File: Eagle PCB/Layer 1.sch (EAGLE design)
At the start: 231 parts, among them M1C1 33nF, M1C2 680uF, M1C3 1.0uF, M1D1 RED, M1D2 BLUE, M1J1 XT30PB-F, M1Q1 AOD482, M1R1 1k, M1R10 1k, M1R11 10k, M1R12 4.7k, M1R2 1k, M1R3 3.3k, M1R4 3.3k, M1R5 1k, M1R6 1k, M1R7 1k, M1R8 10k, M1R9 10k, M2C1 33nF, M2C2 680uF, M2C3 1.0uF, M2D1 RED, M2D2 BLUE, M2J1 XT30PB-F, M2Q1 AOD482, M2R1 1k, M2R10 1k, M2R11 10k, M2R12 4.7k, M2R2 1k, M2R3 3.3k, M2R4 3.3k, M2R5 1k, M2R6 1k, M2R7 1k, M2R8 10k, M2R9 10k, M3C1 33nF, M3C2 680uF, M3C3 1.0uF, M3D1 RED, M3D2 BLUE, M3J1 XT30PB-F, M3Q1 AOD482, M3R1 1k, M3R10 1k, M3R11 10k, M3R12 4.7k, M3R2 1k, M3R3 3.3k, M3R4 3.3k, M3R5 1k, M3R6 1k, M3R7 1k, M3R8 10k, M3R9 10k, M4C1 33nF, M4C2 680uF, M4C3 1.0uF, M4D1 RED, M4D2 BLUE, M4J1 XT30PB-F, M4Q1 AOD482, M4R1 1k, M4R10 1k, M4R11 10k, M4R12 4.7k, M4R2 1k, M4R3 3.3k, M4R4 3.3k, M4R5 1k, M4R6 1k, M4R7 1k, M4R8 10k, M4R9 10k, Q1 LIGHT_SENSORALS, Q10 LIGHT_SENSORALS, Q11 LIGHT_SENSORALS, Q12 LIGHT_SENSORALS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

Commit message: FUCK YOU
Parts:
- added 1C10: 22uF, JH:CAPACITOR1210
- added 1C6: 4.7uF, JH:CAPACITOR0603
- added 1C7: 220uF, SparkFun-Capacitors:100UF-POLAR-EIA7343-10V-10%(TANT)
- added 1C8: 10nF, JH:CAPACITOR0603
- added 1C9: 0.1uF, JH:CAPACITOR0603
- added 1D2: SS54, JH:DIODE-SCHOTTKY
- added 1L2: 10uH, JH:INDUCTORSWPA8040
- added 1R3: 10k, JH:RESISTOR0603
- added 1R4: 3.24k, JH:RESISTOR0603
- added BATT: XT30PB-F, JH:XT30PB-F
- added U2: (no value), JH:TPS54X0
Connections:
- new net 5V: 1C7.+, 1C9.1, 1L2.2, 1R3.2
- new net N$3: 1C8.2, 1D2.C, 1L2.1, U2.PH
- new net N$5: 1R3.1, 1R4.2, U2.VSNS
- new net N$6: 1C8.1, U2.BOOT
- net GND: now also 1C10.2, 1C6.2, 1C7.-, 1C9.2, 1D2.A, 1R4.1, BATT.P$V-, U2.GND
- net V_BATT: now also 1C10.1, 1C6.1, BATT.P$V+, U2.VIN
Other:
- note added: "5V BUCK"

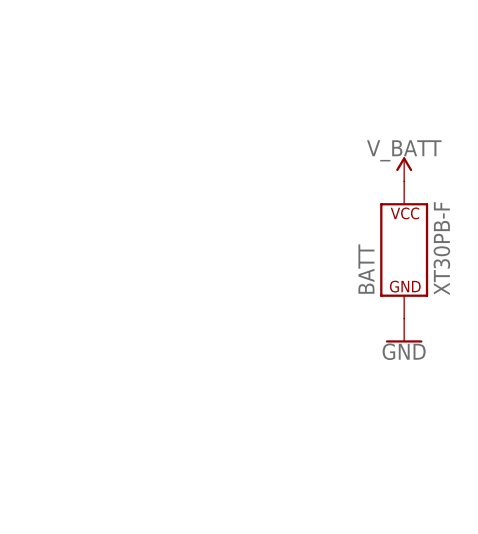
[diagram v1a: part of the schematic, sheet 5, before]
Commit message: Hello
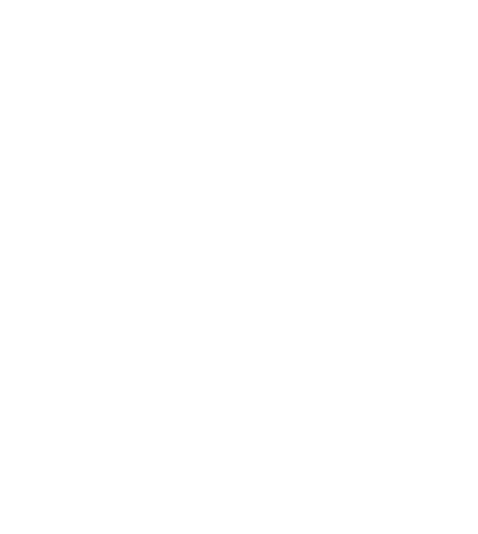
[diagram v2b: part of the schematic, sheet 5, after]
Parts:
- removed BATT: XT30PB-F, JH:XT30PB-F
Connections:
- net GND: no longer BATT.P$V-
- net V_BATT: no longer BATT.P$V+
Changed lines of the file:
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@@
 <part name="V_BATT_M4B" library="JH" library_urn="urn:adsk.eagle:library:6027132" deviceset="18AWG" device="" package3d_urn="urn:adsk.eagle:package:16754415/1"/>
 <part name="FRAME2" library="SparkFun-Aesthetics" deviceset="FRAME-A4L" device=""/>
-<part name="SUPPLY3" library="SparkFun-PowerSymbols" deviceset="V_BATT" device=""/>
-<part name="GND16" library="SparkFun-PowerSymbols" deviceset="GND" device=""/>
 <part name="SUPPLY22" library="SparkFun-PowerSymbols" deviceset="V_BATT" device=""/>
 <part name="1C6" library="JH" library_urn="urn:adsk.eagle:library:6027132" deviceset="CAPACITOR" device="0603" package3d_urn="urn:adsk.eagle:package:15441226/3" value="4.7uF"/>
@@
 <part name="1C9" library="JH" library_urn="urn:adsk.eagle:library:6027132" deviceset="CAPACITOR" device="0603" package3d_urn="urn:adsk.eagle:package:15441226/3" value="0.1uF"/>
 <part name="SUPPLY28" library="SparkFun-PowerSymbols" deviceset="5V" device=""/>
-<part name="BATT" library="JH" library_urn="urn:adsk.eagle:library:6027132" deviceset="XT30" device="PB-F" package3d_urn="urn:adsk.eagle:package:15925142/7"/>
 <part name="1C10" library="JH" library_urn="urn:adsk.eagle:library:6027132" deviceset="CAPACITOR" device="1210" package3d_urn="urn:adsk.eagle:package:15441227/3" value="22uF"/>
 </parts>
@@
 <attribute name="DESIGNER" x="231.34" y="13.97" size="2.54" layer="94" font="vector"/>
 </instance>
-<instance part="SUPPLY3" gate="G$1" x="210.82" y="137.16" smashed="yes">
-<attribute name="VALUE" x="210.82" y="139.954" size="1.778" layer="96" align="bottom-center"/>
-</instance>
-<instance part="GND16" gate="1" x="210.82" y="119.38" smashed="yes">
-<attribute name="VALUE" x="210.82" y="119.126" size="1.778" layer="96" align="top-center"/>
-</instance>
 <instance part="SUPPLY22" gate="G$1" x="50.8" y="149.86" smashed="yes">
 <attribute name="VALUE" x="50.8" y="152.654" size="1.778" layer="96" align="bottom-center"/>
@@
 <attribute name="VALUE" x="129.54" y="150.114" size="1.778" layer="96" align="bottom-center"/>
 </instance>
-<instance part="BATT" gate="G$1" x="210.82" y="129.54" smashed="yes">
-<attribute name="NAME" x="207.518" y="124.46" size="1.778" layer="95" font="vector" rot="R90"/>
-<attribute name="VALUE" x="215.9" y="124.46" size="1.778" layer="95" font="vector" rot="R90"/>
-</instance>
 <instance part="1C10" gate="G$1" x="63.5" y="142.24" smashed="yes">
 <attribute name="NAME" x="65.024" y="144.78" size="1.778" layer="95" font="vector" align="center-left"/>
@@
 <junction x="63.5" y="147.32"/>
 </segment>
-<segment>
-<pinref part="SUPPLY3" gate="G$1" pin="V_BATT"/>
-<pinref part="BATT" gate="G$1" pin="P$V+"/>
-</segment>
 </net>
 <net name="GND" class="0">
@@
 <junction x="139.7" y="119.38"/>
 </segment>
-<segment>
-<pinref part="GND16" gate="1" pin="GND"/>
-<pinref part="BATT" gate="G$1" pin="P$V-"/>
-</segment>
 </net>

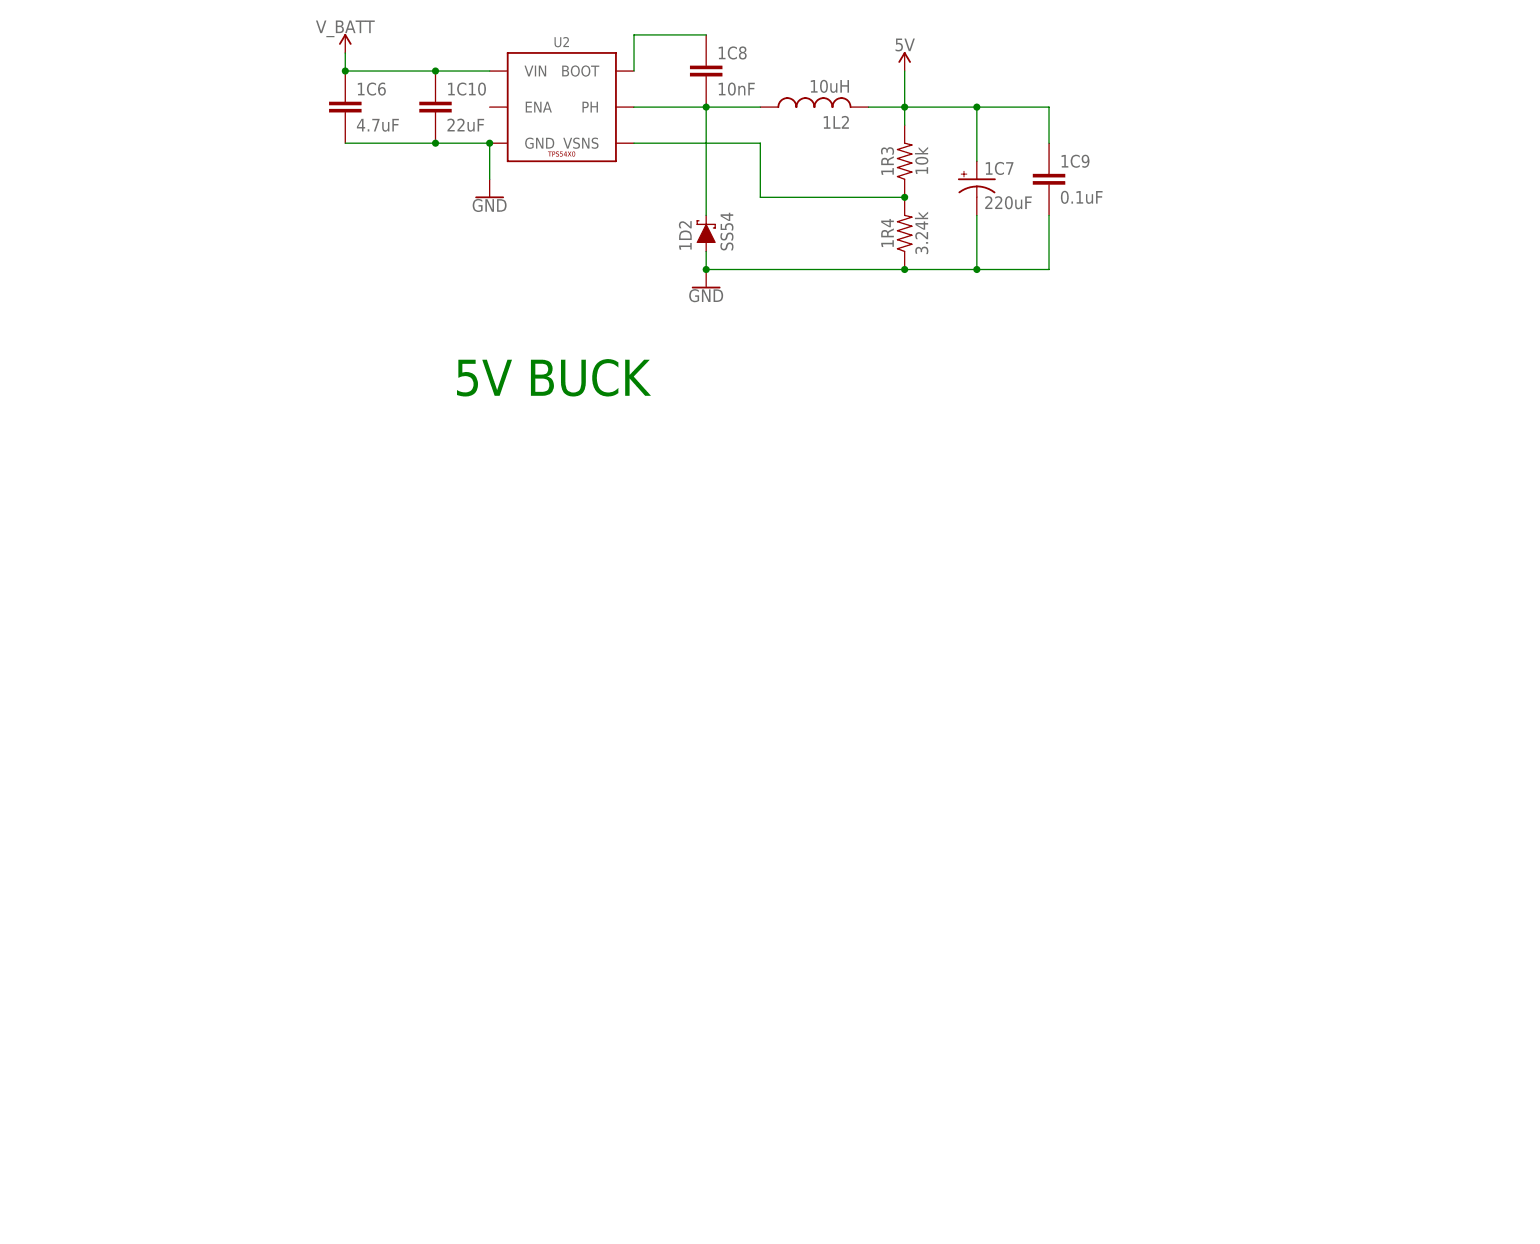
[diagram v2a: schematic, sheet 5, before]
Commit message: macOS
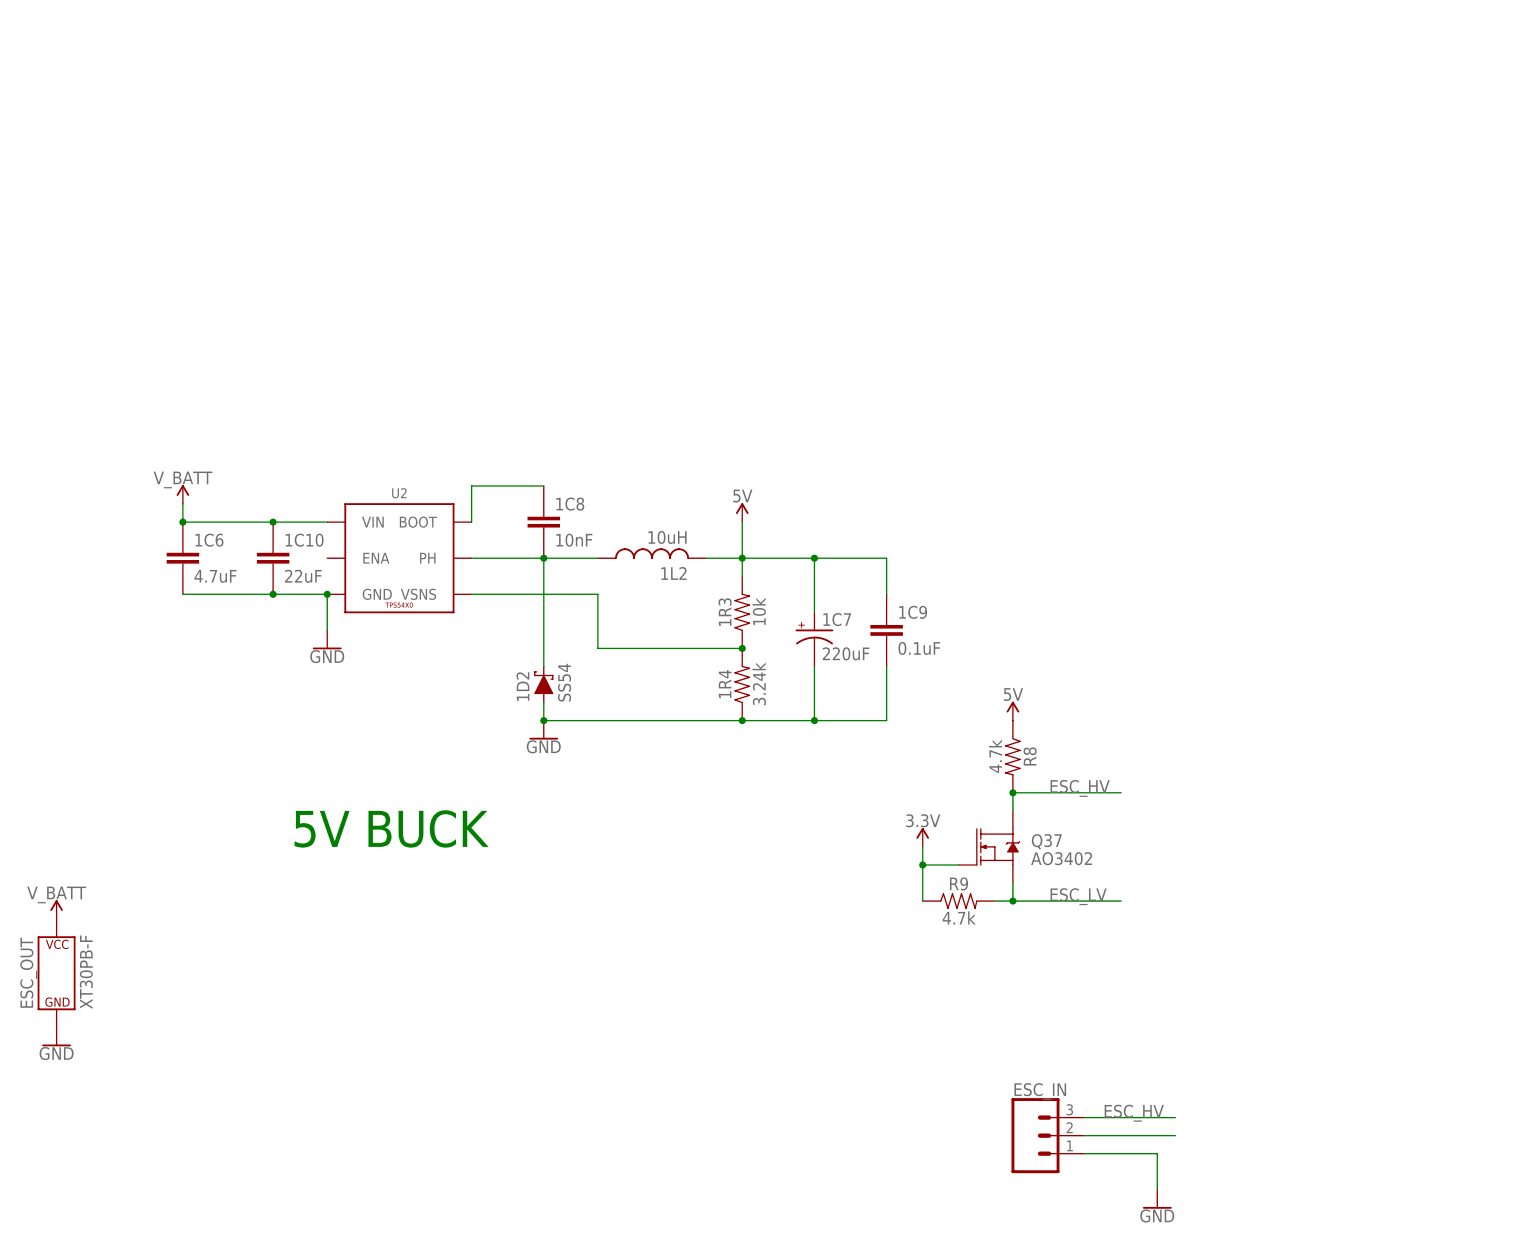
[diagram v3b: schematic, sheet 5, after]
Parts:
- added ESC_IN: (no value), SparkFun-Connectors:CONN_03LOCK
- added ESC_OUT: XT30PB-F, JH:XT30PB-F
- added Q37: AO3402, SparkFun-DiscreteSemi:MOSFET-NCH-AO3404A
- added R8, R9: 4.7k, JH:RESISTOR0603
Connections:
- new net 3.3V1: Q37.G, R9.1
- new net ESC_HV: ESC_IN.3, Q37.D, R8.2
- new net ESC_LV: Q37.S, R9.2
- new net GND1: ESC_IN.1
- new net N$7: ESC_IN.2
- net 5V: now also R8.1
- net GND: now also ESC_OUT.P$V-
- net V_BATT: now also ESC_OUT.P$V+
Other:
- moved on the sheet: 1C10, 1C6, 1C7, 1C8, 1C9, 1D2, 1L2, 1R3, 1R4, U2

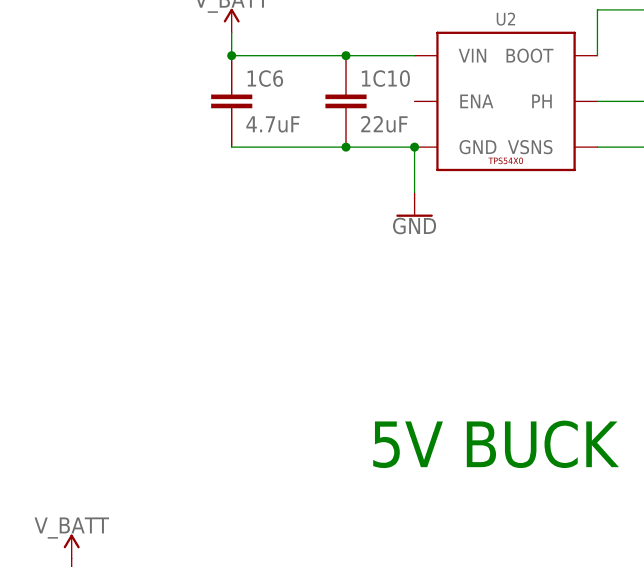
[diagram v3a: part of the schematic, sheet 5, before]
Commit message: Done
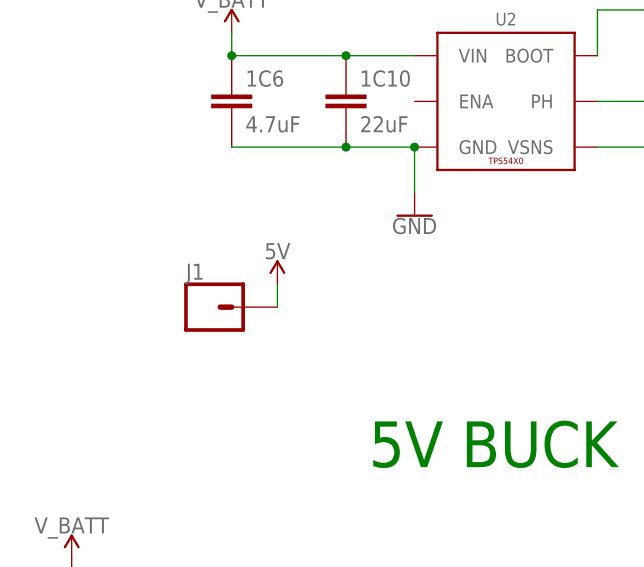
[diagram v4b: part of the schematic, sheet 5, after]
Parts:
- added J1: (no value), Connectors:CONN_01
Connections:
- removed net GND1: ESC_IN.1
- net 5V: now also J1.1
- net GND: now also ESC_IN.1
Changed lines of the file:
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@@
 <part name="SUPPLY31" library="SparkFun-PowerSymbols" deviceset="5V" device=""/>
 <part name="SUPPLY32" library="SparkFun-PowerSymbols" deviceset="3.3V" device=""/>
-<part name="GND39" library="SparkFun-PowerSymbols" deviceset="GND" device=""/>
 <part name="ESC_IN" library="SparkFun-Connectors" library_urn="urn:adsk.eagle:library:11010760" deviceset="CONN_03" device="LOCK" package3d_urn="urn:adsk.eagle:package:11011273/2"/>
+<part name="J1" library="Connectors" library_urn="urn:adsk.eagle:library:19813715" deviceset="CONN_01" device="" package3d_urn="urn:adsk.eagle:package:19813825/2"/>
+<part name="SUPPLY33" library="SparkFun-PowerSymbols" deviceset="5V" device=""/>
+<part name="GND39" library="SparkFun-PowerSymbols" deviceset="GND" device=""/>
 </parts>
 <sheets>
@@
 <attribute name="VALUE" x="132.08" y="40.894" size="1.778" layer="96" align="bottom-center"/>
 </instance>
-<instance part="GND39" gate="1" x="165.1" y="-12.7" smashed="yes">
-<attribute name="VALUE" x="165.1" y="-12.954" size="1.778" layer="96" align="top-center"/>
-</instance>
 <instance part="ESC_IN" gate="J$1" x="147.32" y="-2.54" smashed="yes">
 <attribute name="VALUE" x="144.78" y="-9.906" size="1.778" layer="96" font="vector"/>
 <attribute name="NAME" x="144.78" y="3.048" size="1.778" layer="95" font="vector"/>
 </instance>
+<instance part="J1" gate="G$1" x="25.4" y="55.88" smashed="yes">
+<attribute name="VALUE" x="22.86" y="51.054" size="1.778" layer="96" font="vector"/>
+<attribute name="NAME" x="22.86" y="58.928" size="1.778" layer="95" font="vector"/>
+</instance>
+<instance part="SUPPLY33" gate="G$1" x="33.02" y="58.42" smashed="yes">
+<attribute name="VALUE" x="33.02" y="61.214" size="1.778" layer="96" align="bottom-center"/>
+</instance>
+<instance part="GND39" gate="1" x="165.1" y="-12.7" smashed="yes">
+<attribute name="VALUE" x="165.1" y="-12.954" size="1.778" layer="96" align="top-center"/>
+</instance>
 </instances>
 <busses>
@@
 <pinref part="ESC_OUT" gate="G$1" pin="P$V-"/>
 </segment>
+<segment>
+<wire x1="154.94" y1="-5.08" x2="165.1" y2="-5.08" width="0.1524" layer="91"/>
+<wire x1="165.1" y1="-5.08" x2="165.1" y2="-10.16" width="0.1524" layer="91"/>
+<pinref part="ESC_IN" gate="J$1" pin="1"/>
+<pinref part="GND39" gate="1" pin="GND"/>
+</segment>
 </net>
 <net name="N$3" class="0">
@@
 <pinref part="R8" gate="G$1" pin="1"/>
 </segment>
+<segment>
+<pinref part="J1" gate="G$1" pin="1"/>
+<pinref part="SUPPLY33" gate="G$1" pin="5V"/>
+<wire x1="33.02" y1="58.42" x2="33.02" y2="55.88" width="0.1524" layer="91"/>
+</segment>
 </net>
 <net name="ESC_HV" class="0">
@@
 </segment>
 </net>
-<net name="GND1" class="0">
-<segment>
-<wire x1="154.94" y1="-5.08" x2="165.1" y2="-5.08" width="0.1524" layer="91"/>
-<wire x1="165.1" y1="-5.08" x2="165.1" y2="-10.16" width="0.1524" layer="91"/>
-<pinref part="GND39" gate="1" pin="GND"/>
-<pinref part="ESC_IN" gate="J$1" pin="1"/>
-</segment>
-</net>
